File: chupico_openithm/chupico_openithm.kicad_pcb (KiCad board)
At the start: 2 copper layers, 100 x 55.1 mm, 25 parts, among them J1 Conn_01x06, J10 Conn_02x12_Odd_Even, J11 Conn_02x12_Odd_Even, J2 Conn_01x12, J3 Conn_01x06, J4 Conn_01x12, J5 Conn_01x06, J6 Conn_01x12, J7 Conn_01x08, J8 Conn_01x11, J9 Conn_01x11, U1 Pico

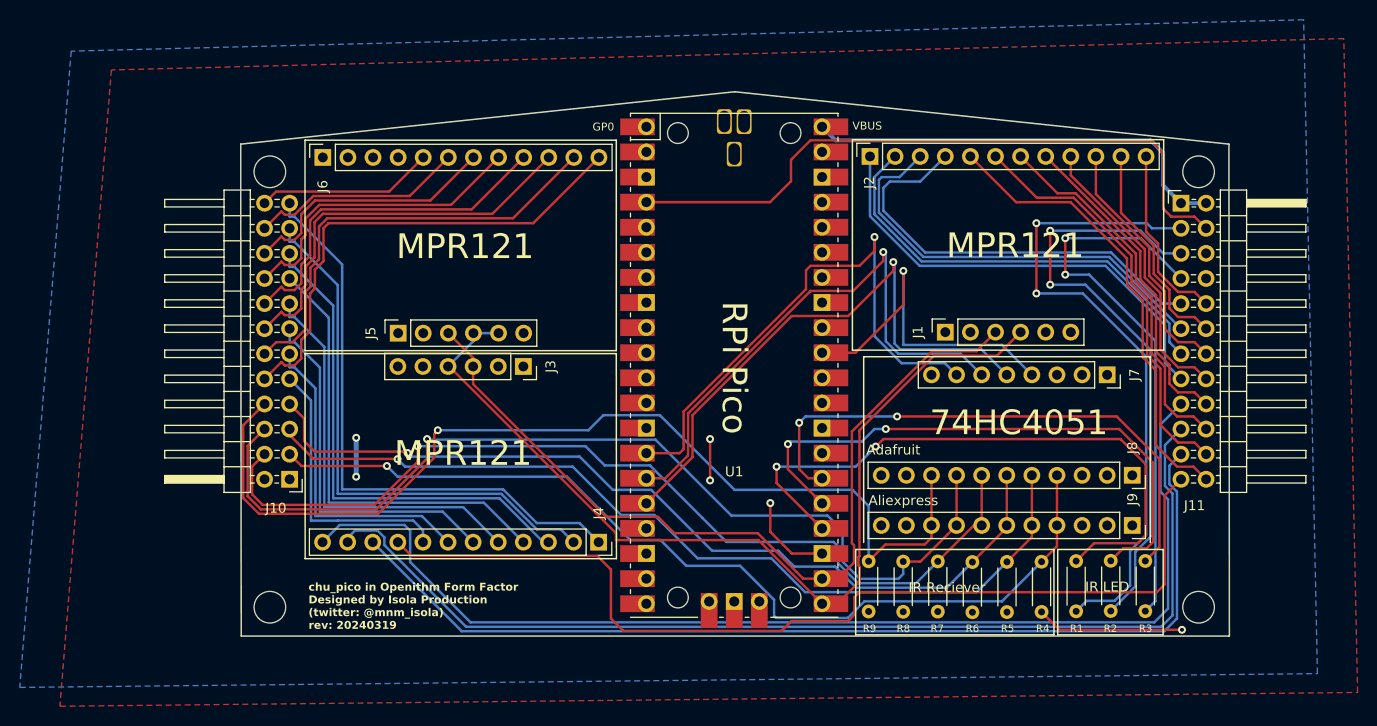
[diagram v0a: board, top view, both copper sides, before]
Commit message: Update README.md
Update README.md
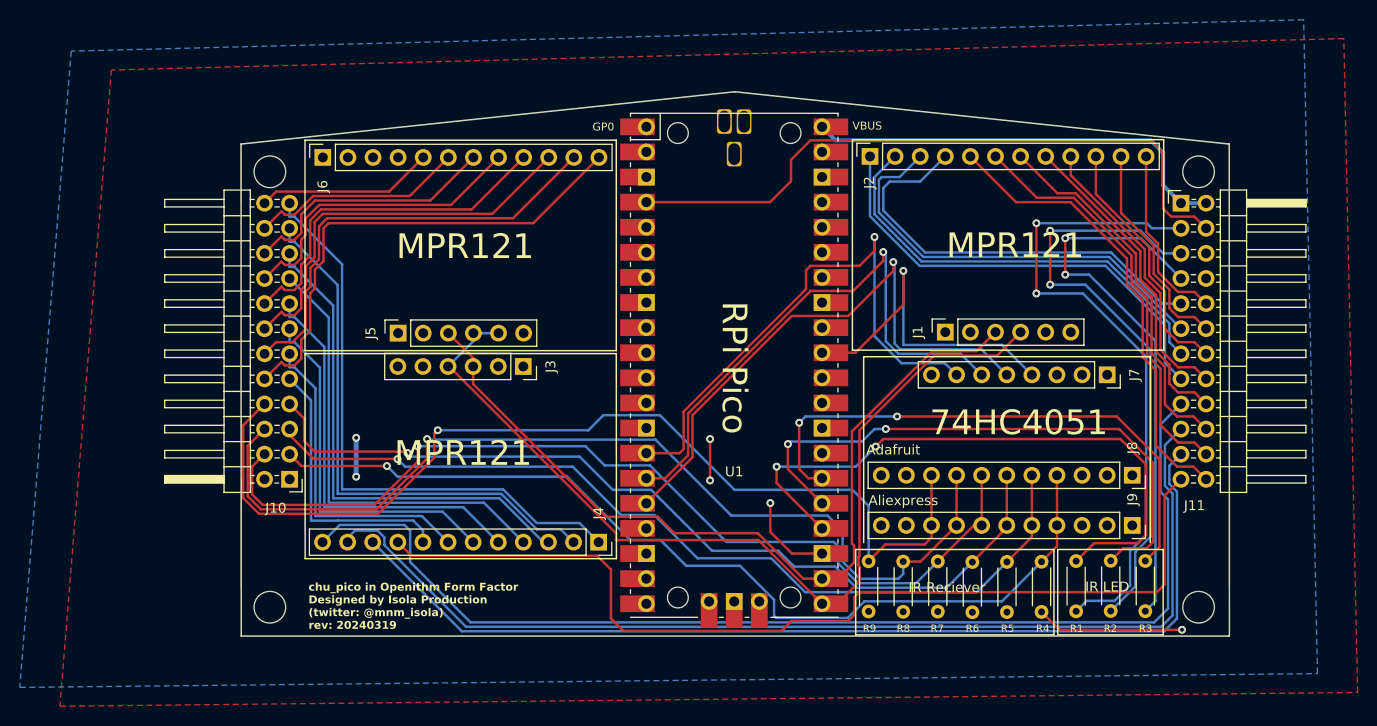
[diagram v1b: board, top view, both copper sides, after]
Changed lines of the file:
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@@
   (gr_line (start 183.57 81.556) (end 152.07 81.556)
     (stroke (width 0.15) (type solid)) (layer "F.SilkS"))
-  (gr_rect (start 183.515 101.727) (end 172.847 110.363)
+  (gr_rect (start 172.847 101.727) (end 183.515 110.363)
     (stroke (width 0.15) (type default)) (fill none) (layer "F.SilkS"))
   (gr_line (start 128.175 60.306) (end 128.175 81.606)
@@
   (gr_line (start 152.07 60.256) (end 183.57 60.256)
     (stroke (width 0.15) (type solid)) (layer "F.SilkS"))
-  (gr_line (start 90.17 60.706) (end 90.22 110.49)
+  (gr_line (start 90.2 60.7) (end 90.22 110.49)
     (stroke (width 0.15) (type solid)) (layer "Edge.Cuts"))
-  (gr_line (start 190.22 110.49) (end 190.17 60.706)
+  (gr_line (start 190.22 110.49) (end 190.2 60.7)
     (stroke (width 0.15) (type solid)) (layer "Edge.Cuts"))
-  (gr_line (start 140.17 55.406) (end 90.17 60.706)
+  (gr_line (start 140.17 55.406) (end 90.2 60.7)
     (stroke (width 0.15) (type solid)) (layer "Edge.Cuts"))
   (gr_line (start 90.22 110.49) (end 190.22 110.49)
     (stroke (width 0.15) (type solid)) (layer "Edge.Cuts"))
-  (gr_line (start 140.17 55.406) (end 190.17 60.706)
+  (gr_line (start 140.17 55.406) (end 190.2 60.7)
     (stroke (width 0.15) (type solid)) (layer "Edge.Cuts"))
   (gr_text "chu_pico in Openithm Form Factor\nDesigned by Isola Production\n(twitter: @mnm_isola)\nrev: 20240319" (at 97.028 109.855) (layer "F.SilkS")
